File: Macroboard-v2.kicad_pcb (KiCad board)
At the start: 2 copper layers, 7 parts, among them SW1 SW_Push, SW2 SW_Push, SW3 SW_Push, SW4 SW_Push, U1 XIAO-RP2040-DIP

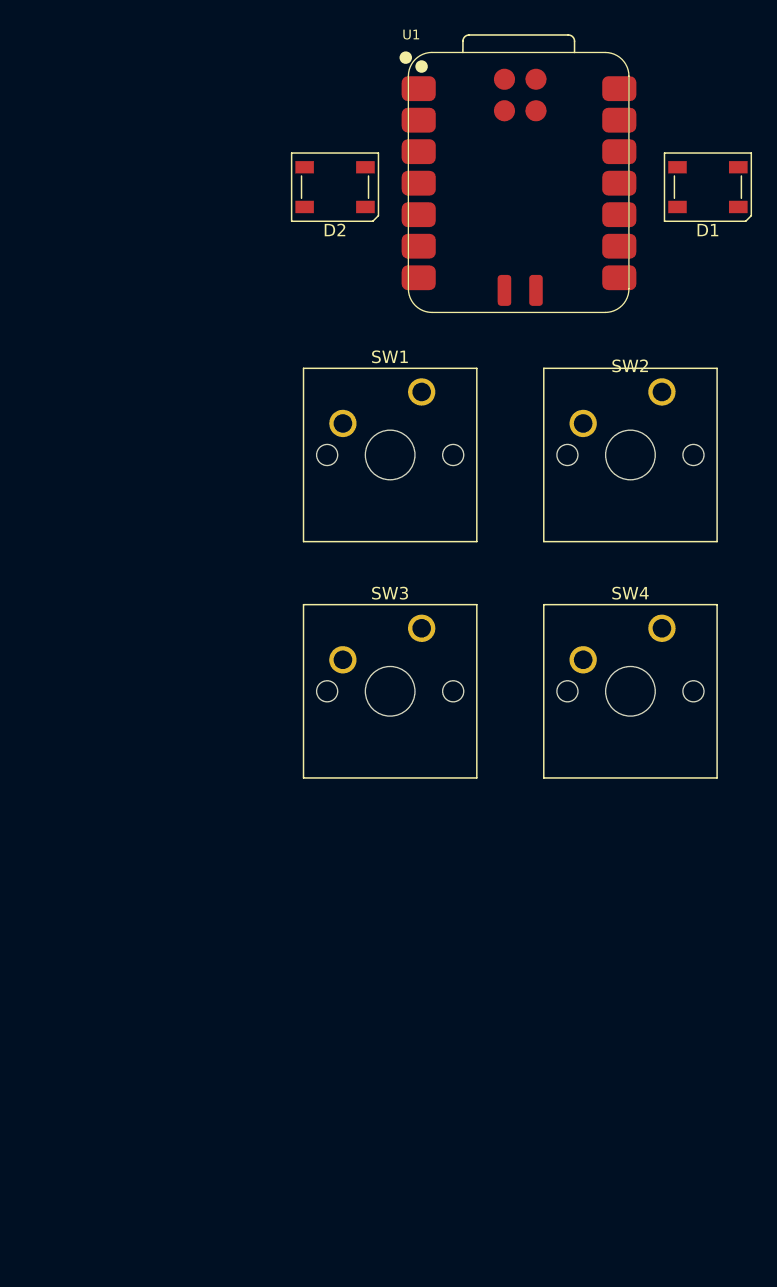
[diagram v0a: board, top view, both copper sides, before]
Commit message: 20:49 - 2025-5-21
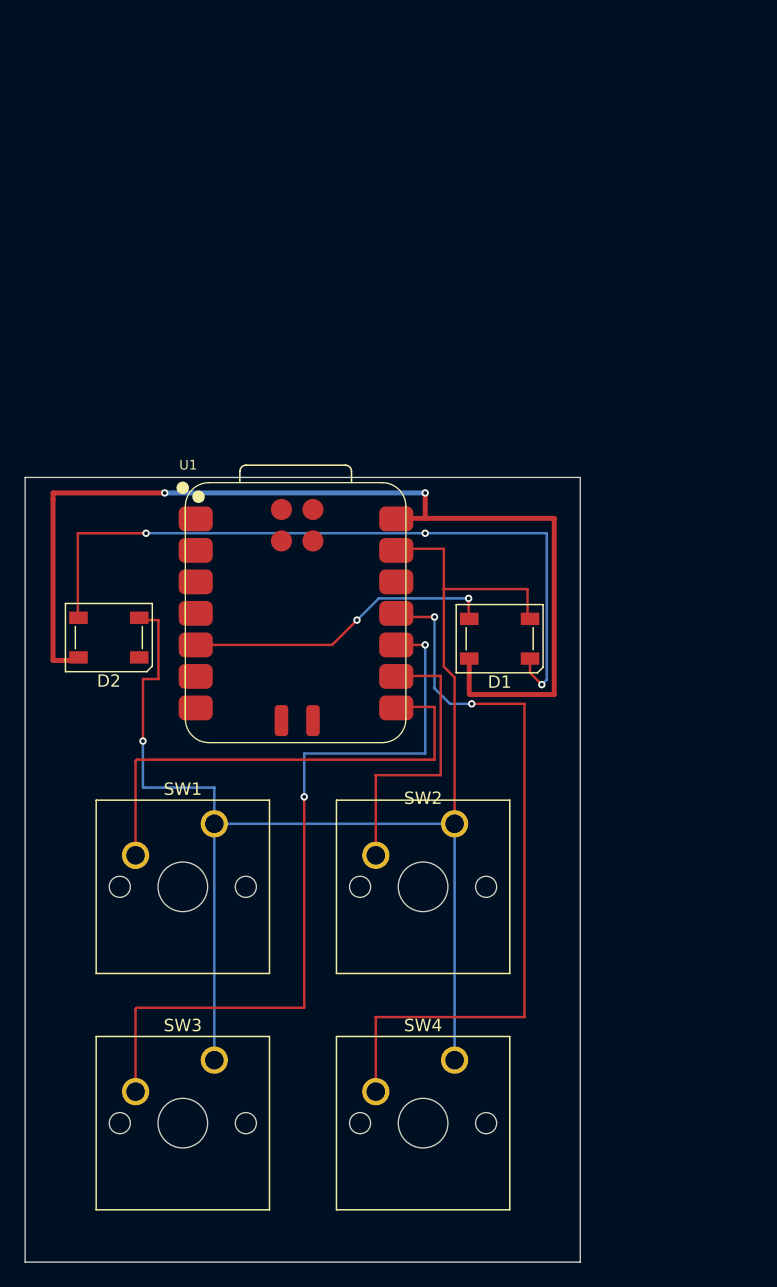
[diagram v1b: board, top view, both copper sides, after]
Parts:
- moved D2 40.6 mm to (156.5, 74.4)
- moved D1 40.1 mm to (188.0, 74.5)
- moved U1 39.1 mm to (171.5, 72.5)
- moved SW1 38.6 mm to (165.0, 89.4)
- moved SW2 38.6 mm to (184.4, 89.4)
- moved SW3 38.6 mm to (165.0, 108.5)
- moved SW4 38.6 mm to (184.4, 108.5)
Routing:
- net GND: track 0.00 -> 118.2 mm, vias 0 -> 1
- net +5V: track 0.00 -> 84.4 mm, vias 0 -> 2
- net Net-(U1-GPIO4/MISO): track 0.00 -> 61.6 mm, vias 0 -> 2
- net Net-(U1-GPIO3/MOSI): track 0.00 -> 60.0 mm, vias 0 -> 2
- net Net-(D1-VSS): track 0.00 -> 59.3 mm, vias 0 -> 3
- net Net-(U1-GPIO1/RX): track 0.00 -> 39.1 mm
- net Net-(D1-VDD): track 0.00 -> 25.2 mm, vias 0 -> 2
- net Net-(U1-GPIO2/SCK): track 0.00 -> 23.3 mm
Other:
- board outline added: 44.8 x 63.2 mm
